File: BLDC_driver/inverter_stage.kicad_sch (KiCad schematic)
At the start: 66 parts, among them Q1 AOTL66912, Q2 AOTL66912, Q3 AOTL66912, Q4 AOTL66912, Q5 AOTL66912, Q6 AOTL66912

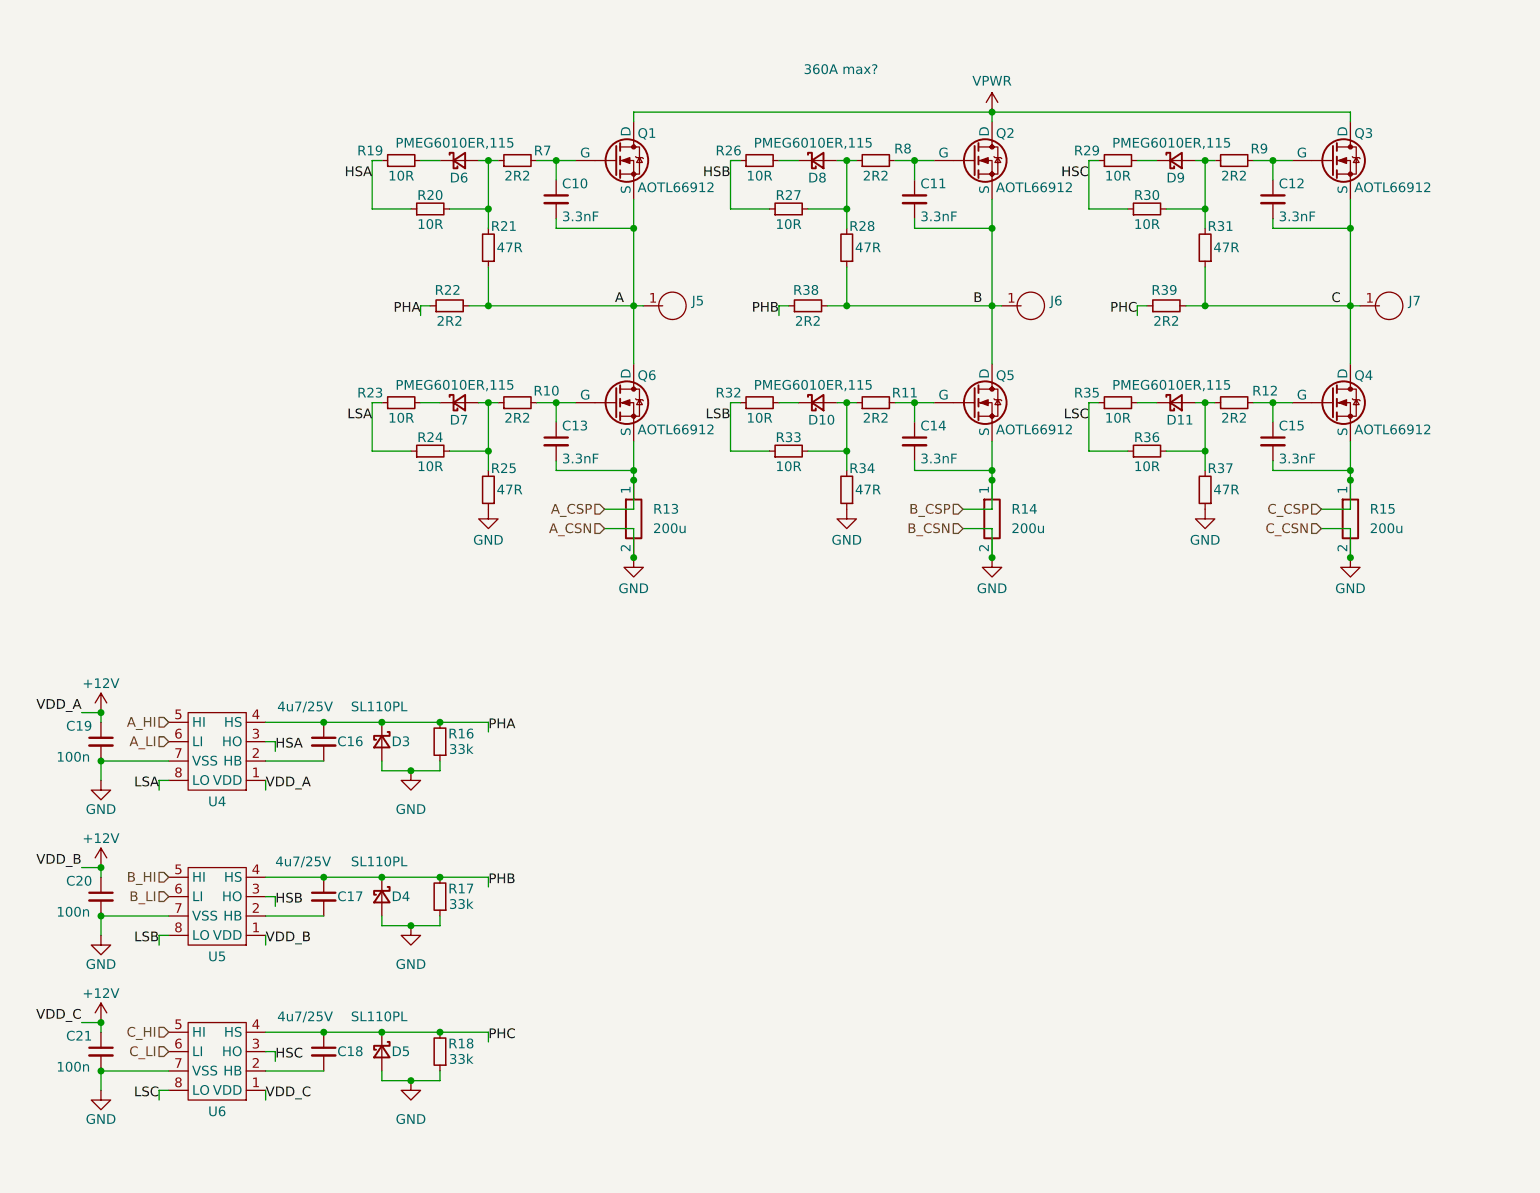
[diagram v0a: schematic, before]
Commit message: New design
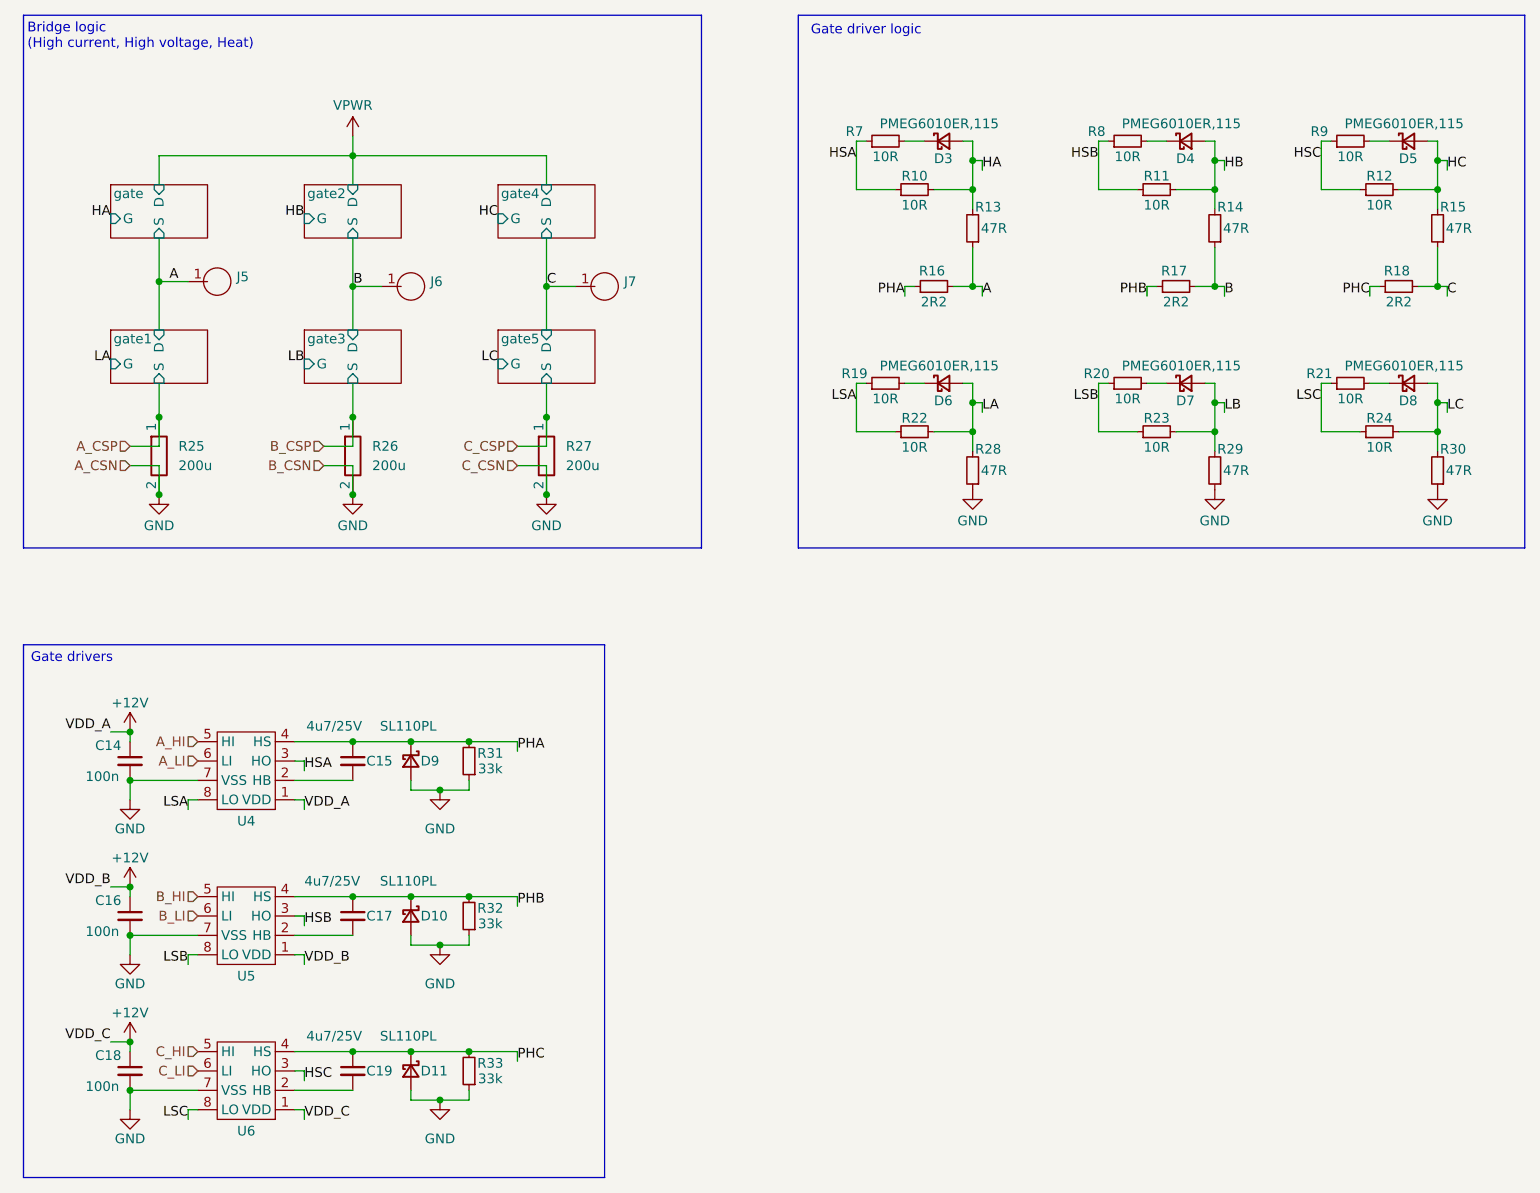
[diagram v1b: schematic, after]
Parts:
- removed C10, C11, C12, C13, C14, C15: 3.3nF, Capacitor_SMD:C_0805_2012Metric, symbol Device:C_Small
- removed Q1, Q2, Q3, Q4, Q5, Q6: AOTL66912, Package_TO_SOT_SMD:Infineon_PG-HSOF-8-1_ThermalVias, symbol Marijn:AOTL66912
- removed R10, R11, R12, R7, R8, R9: 2R2, Resistor_SMD:R_0603_1608Metric, symbol Device:R_Small
- renumbered C19 to C14, C16 to C15, C20 to C16, C21 to C18, C18 to C19, D4 to D10, D5 to D11, D6 to D3, D8 to D4, D9 to D5, D7 to D6, D10 to D7, D11 to D8, D3 to D9, R20 to R10, R27 to R11, R30 to R12, R21 to R13, R28 to R14, R31 to R15, R22 to R16, R38 to R17, R39 to R18, R23 to R19, R32 to R20, R35 to R21, R24 to R22, R33 to R23, R36 to R24, R13 to R25, R14 to R26, R15 to R27, R25 to R28, R34 to R29, R37 to R30, R16 to R31, R17 to R32, R18 to R33, R19 to R7, R26 to R8, R29 to R9
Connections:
- net HA: now reaches D3.2 (A), R10.2, R13.2
- net LB: now reaches D7.2 (A), R23.2, R29.2
- net LA: now reaches D6.2 (A), R22.2, R28.2
- net LC: now reaches D8.2 (A), R24.2, R30.2
- net HC: now reaches D5.2 (A), R12.2, R15.2
- net HB: now reaches D4.2 (A), R11.2, R14.2
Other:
- added sheet gate (gate.kicad_sch)
- added sheet gate1 (gate.kicad_sch)
- added sheet gate2 (gate.kicad_sch)
- added sheet gate3 (gate.kicad_sch)
- added sheet gate4 (gate.kicad_sch)
- added sheet gate5 (gate.kicad_sch)
- note added: "Bridge logic (High current, High voltage, Heat)"
- note added: "Gate driver logic"
- note added: "Gate drivers"
- note removed: "360A max?"
- moved on the sheet: C14, C15, C16, C17, C18, C19, D10, D11, D3, D4, D5, D6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
